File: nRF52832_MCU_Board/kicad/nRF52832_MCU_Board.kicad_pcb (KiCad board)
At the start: 2 copper layers, 65 x 40 mm, 60 parts, among them J1 CONN_01X03, J2 CONN_01X16, J3 CONN_01X08, J4 CONN_01X03, J5 MICROUSB, J6 CONN_02X05, J7 CONN_01X05, J8 MM8130-2600, J9 CONN_01X08, U2 TLV1117, X1 32MHz, X2 32.768kHz

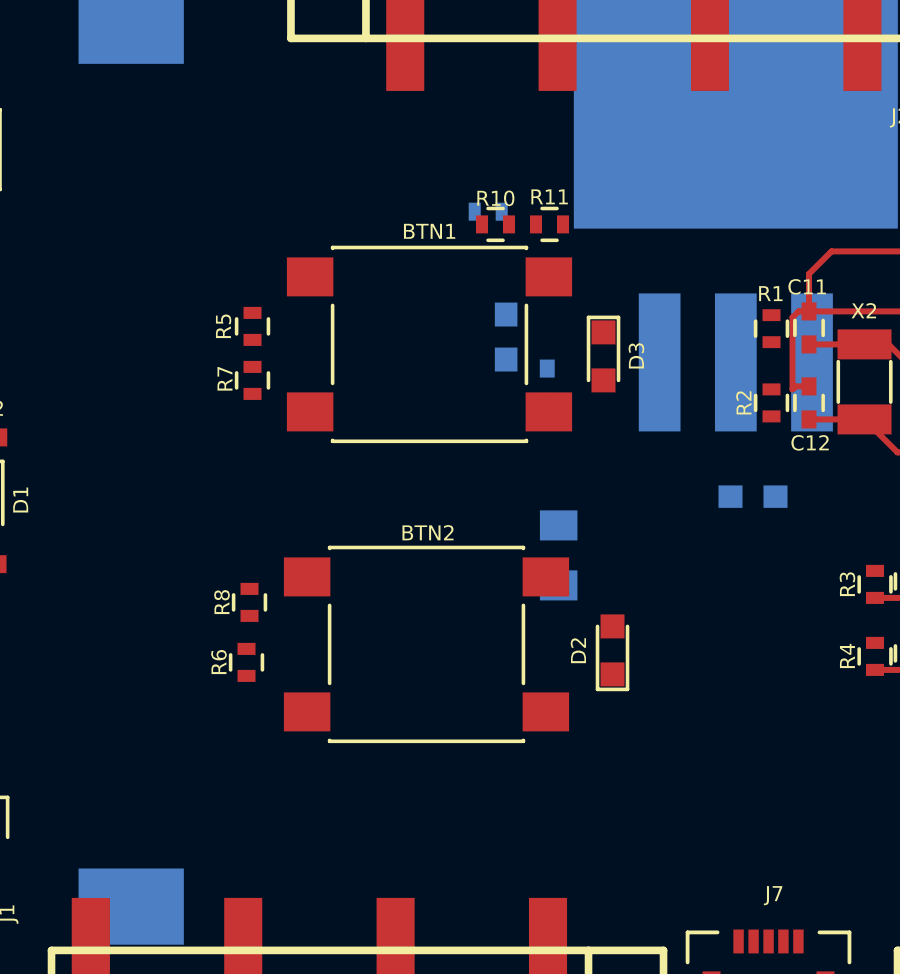
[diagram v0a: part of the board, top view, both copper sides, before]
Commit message: Update KiCAD Project nRF52832_MCU_Board
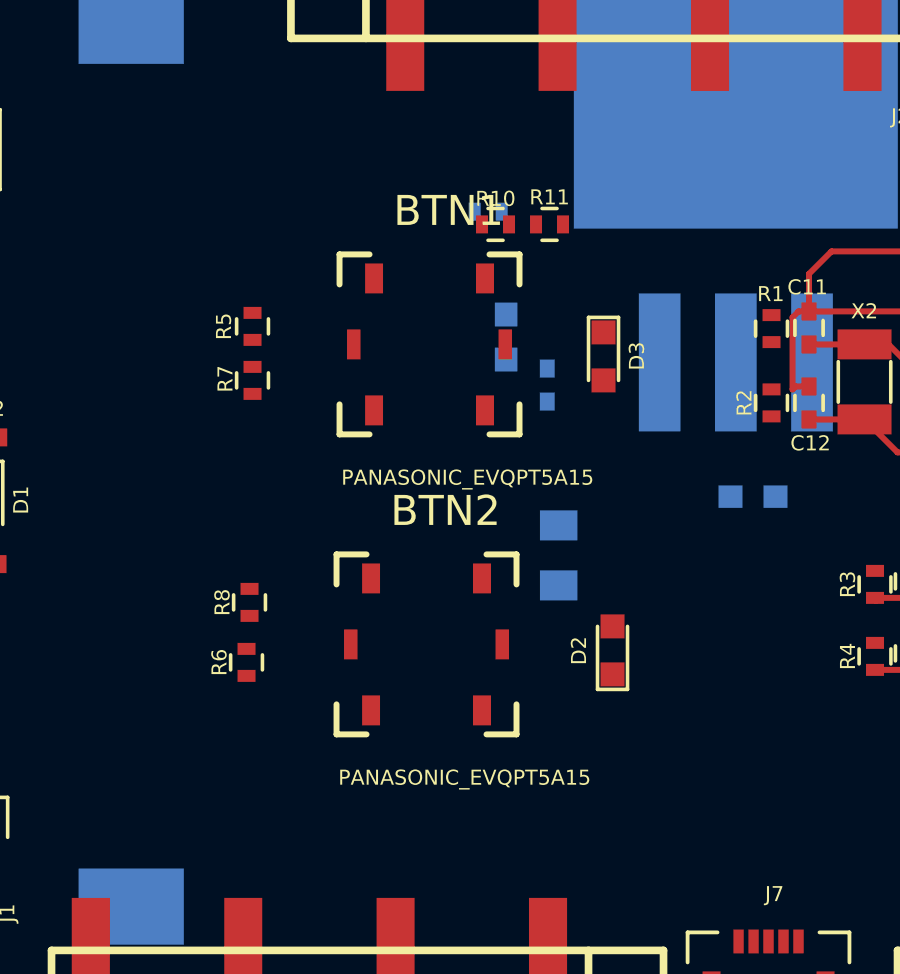
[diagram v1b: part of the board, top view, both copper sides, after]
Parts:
- BTN1, BTN2: footprint Buttons_Switches_SMD:SW_SPST_PTS645 -> Nordic_misc:Nordic_misc-PANASONIC_EVQPT5A15
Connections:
- BTN2 pad 2: Net-(BTN2-Pad2) -> (no net)
